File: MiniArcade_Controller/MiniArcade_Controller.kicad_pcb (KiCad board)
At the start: 2 copper layers, 55 x 25 mm, 7 parts, among them J1 Conn_01x05_Pin, J2 Conn_01x05_Pin, SW1 SW_Push_Dual_x2, SW2 SW_Push_Dual_x2, SW3 SW_Push_Dual_x2, SW4 SW_Push_Dual_x2

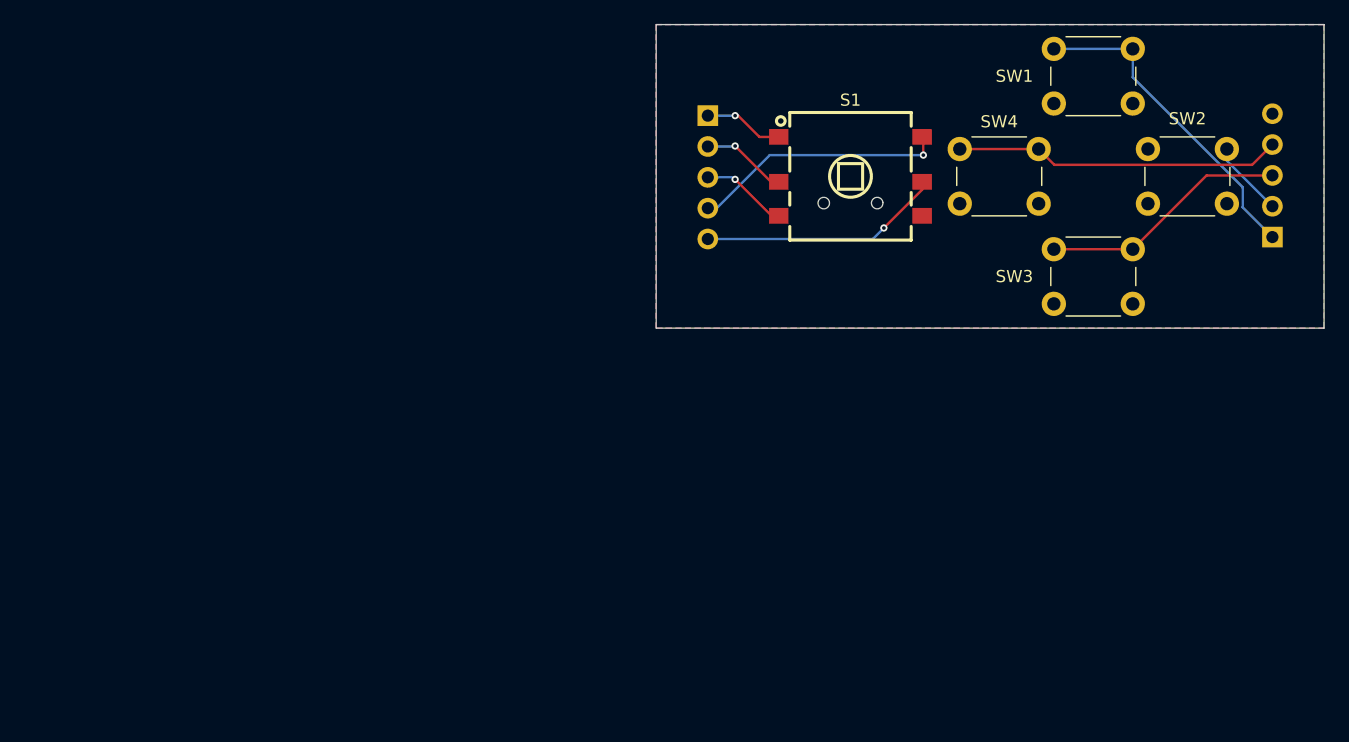
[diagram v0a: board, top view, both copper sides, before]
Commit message: 12 11 2025
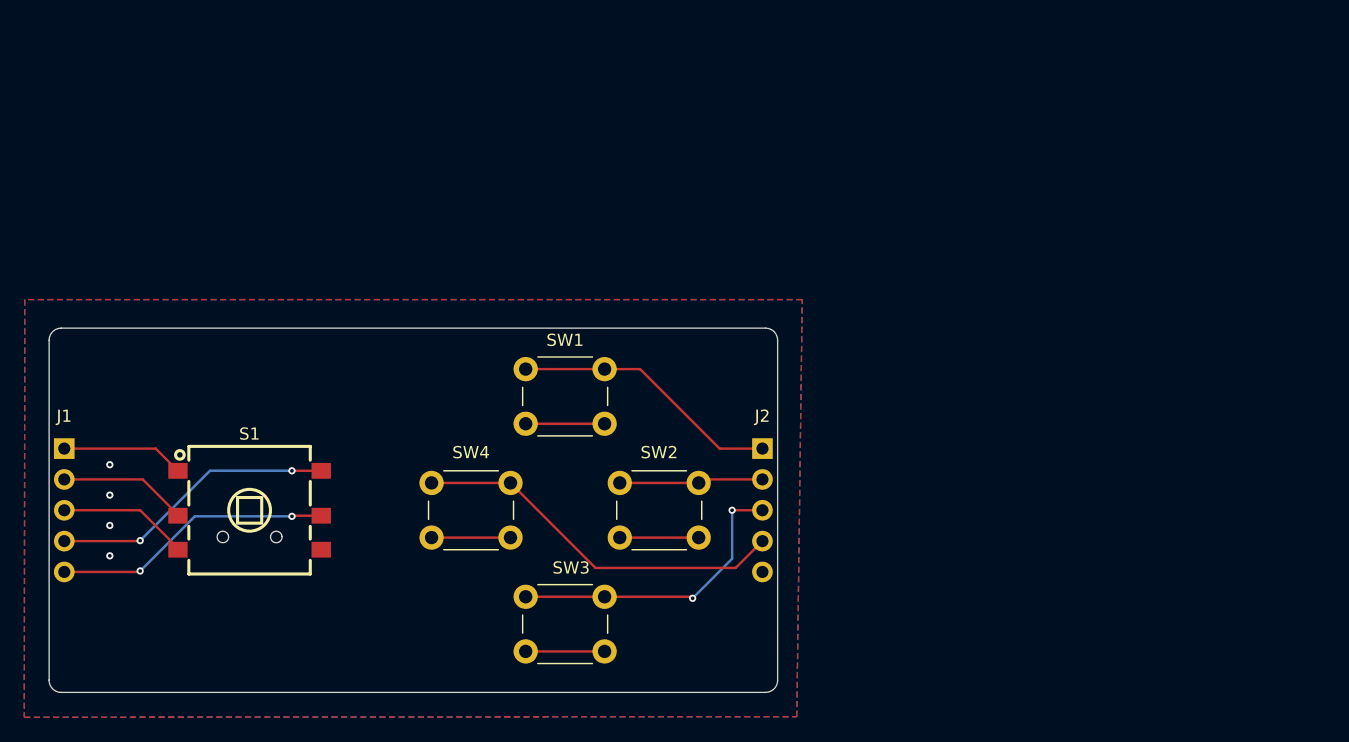
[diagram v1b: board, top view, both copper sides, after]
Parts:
- J1, J2: footprint Connector_PinHeader_2.54mm:PinHeader_1x05_P2.54mm_Horizontal -> Connector_PinHeader_2.54mm:PinHeader_1x05_P2.54mm_Vertical
- moved J1 59.7 mm to (101.2, 109.9)
- moved S1 56.6 mm to (116.5, 115.0)
- moved SW3 52.1 mm to (139.2, 122.1)
- moved SW2 51.5 mm to (147.0, 112.8)
- moved SW4 51.5 mm to (131.5, 112.8)
- moved SW1 50.9 mm to (139.2, 103.4)
- moved J2 45.5 mm to (158.8, 109.9), turned to 180 degrees
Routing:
- net GND: track 0.00 -> 26.0 mm, vias 0 -> 4
- net DP_RIGHT: track 6.26 -> 11.9 mm
- net DP_UP: track 27.1 -> 22.2 mm
- net DP_DOWN: track 20.5 -> 24.9 mm, vias 0 -> 2
- net DP_LEFT: track 27.0 -> 31.1 mm
- net JS_DOWN: track 7.16 -> 10.8 mm, vias 1 -> 0
- net JS_LEFT: track 7.09 -> 10.7 mm, vias 1 -> 0
- net JS_UP: track 6.57 -> 10.1 mm, vias 1 -> 0
- net JS_RIGHT: track 20.0 -> 23.1 mm, vias 1 -> 2
- net JS_SWITCH: track 21.1 -> 23.6 mm, vias 1 -> 2
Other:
- board size 55 x 25 mm -> 60 x 30 mm
